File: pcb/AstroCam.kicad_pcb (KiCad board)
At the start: 2 copper layers, 40 x 40 mm, 93 parts, among them P1 CONN_01X02, P10 CONN_01X14, P2 CONN_01X18, P3 CONN_01X18, P4 CONN_01X04, P5 CONN_01X01, P8 CONN_01X06, P9 CONN_01X02, Q1 2SC5095, Q2 MT3S20TU, Q3 2SC5095, Q4 MT3S20TU, U1 TPS2420, U10 ICX825AQA, U11 ADDI7013, U2 LT3487, U3 TPS63002, U4 TXB0104, U7 TPS56x200, U8 LMZ10500, U9 CXD3400N

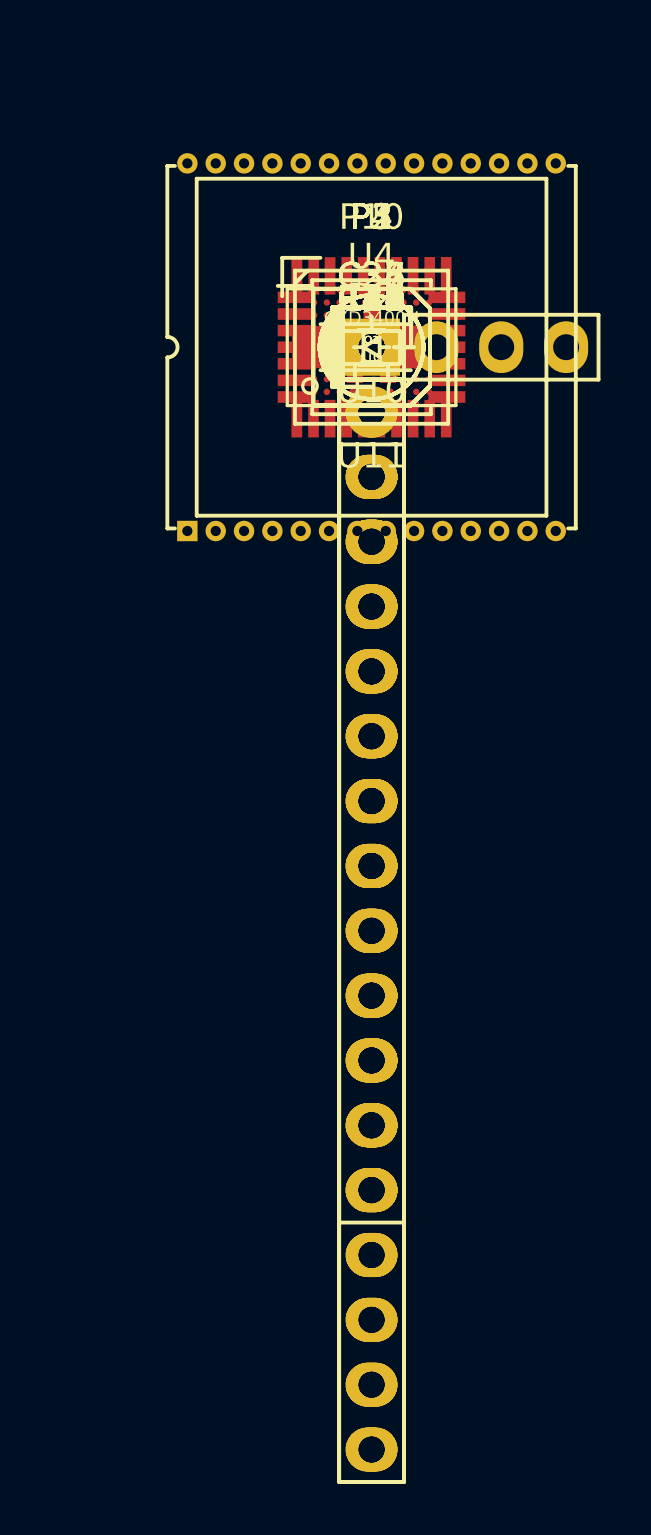
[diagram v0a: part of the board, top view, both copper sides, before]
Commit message: Cleanups
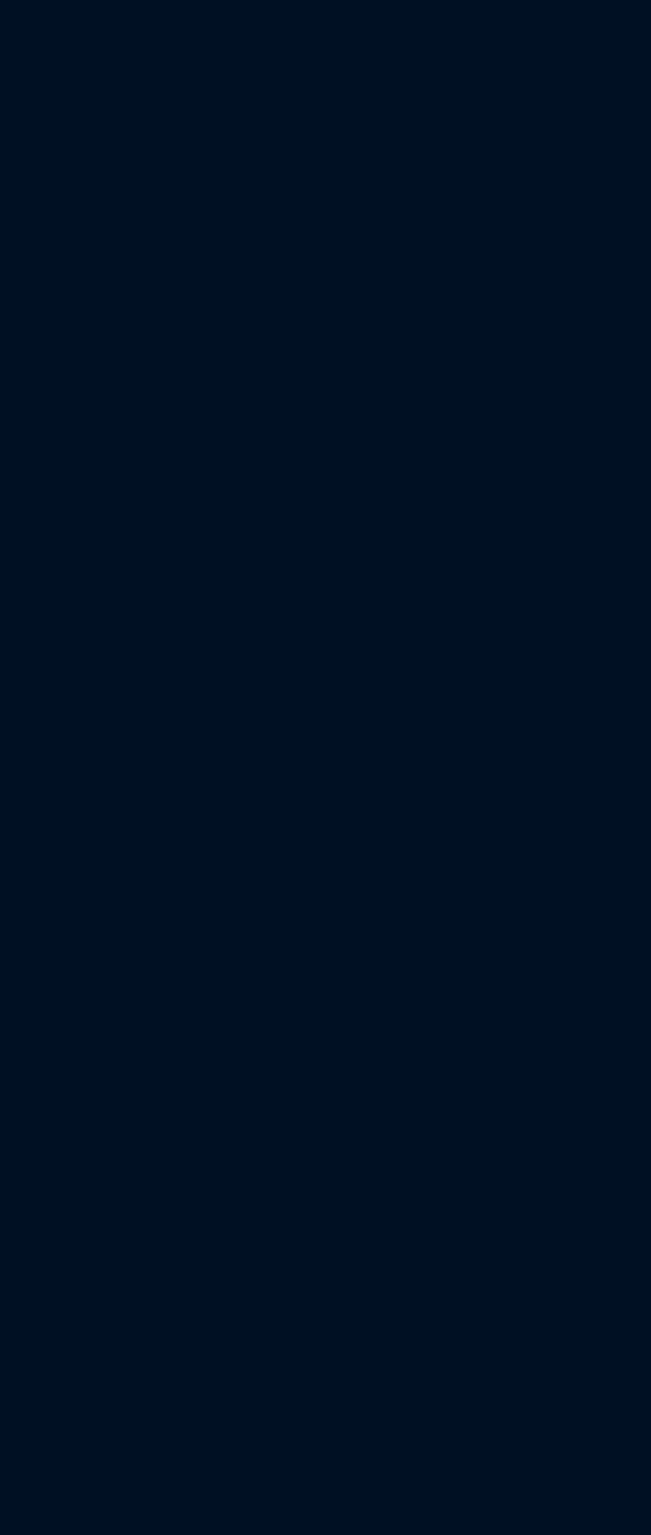
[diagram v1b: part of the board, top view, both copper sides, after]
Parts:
- removed C12, C13, C26, C27: 0.1u, Capacitors_SMD:C_0603
- removed C28: 1u/35V, Capacitors_SMD:c_elec_4x5.3
- removed C29: 0.1uF, Capacitors_SMD:C_0603
- removed C30: 2200pF, Capacitors_SMD:C_0603
- removed C31, C32: 0.1, Capacitors_SMD:C_0603
- removed C33, C35: 0.01, Capacitors_SMD:C_0603
- removed C34, C36, C37: 3.3/20V, Capacitors_SMD:c_elec_4x5.3
- removed C38, C39, C40, C41, C42, C43, C44, C45, C46: 0.1uF, Capacitors_SMD:C_0603_HandSoldering
- removed C47: 4.7uF, Capacitors_SMD:C_0603_HandSoldering
- removed C48, C49: 0.1u, Capacitors_SMD:C_0603_HandSoldering
- removed D2: D, Diodes_SMD:SOD-123
- removed P1: CONN_01X02, Pin_Headers:Pin_Header_Straight_1x02
- removed P10: CONN_01X14, Pin_Headers:Pin_Header_Straight_1x14
- removed P2, P3: CONN_01X18, Pin_Headers:Pin_Header_Straight_1x18
- removed P4: CONN_01X04, Socket_Strips:Socket_Strip_Straight_1x04
- removed P5: CONN_01X01, Socket_Strips:Socket_Strip_Straight_1x01
- removed Q1, Q3: 2SC5095, w_smd_trans:sot323
- removed Q2, Q4: MT3S20TU, w_smd_trans:sot323
- removed R10, R11, R14, R15: 10K, Resistors_SMD:R_0603_HandSoldering
- removed R12, R20: 1.17K, Resistors_SMD:R_0603_HandSoldering
- removed R13, R21: 1.74K, Resistors_SMD:R_0603_HandSoldering
- removed R18: 100k, Resistors_SMD:R_0603_HandSoldering
- removed R19: 1M0, Resistors_SMD:R_0603_HandSoldering
- removed R22: 10.0k, Resistors_SMD:R_0603_HandSoldering
- removed U10: ICX825AQA, camera:ICX825
- removed U11: ADDI7013, camera:csp-bga-bc-76-3
- removed U4: TXB0104, Housings_SSOP:TSSOP-14_4.4x5mm_Pitch0.65mm
- removed U9: CXD3400N, w_smd_dil:tssop-20

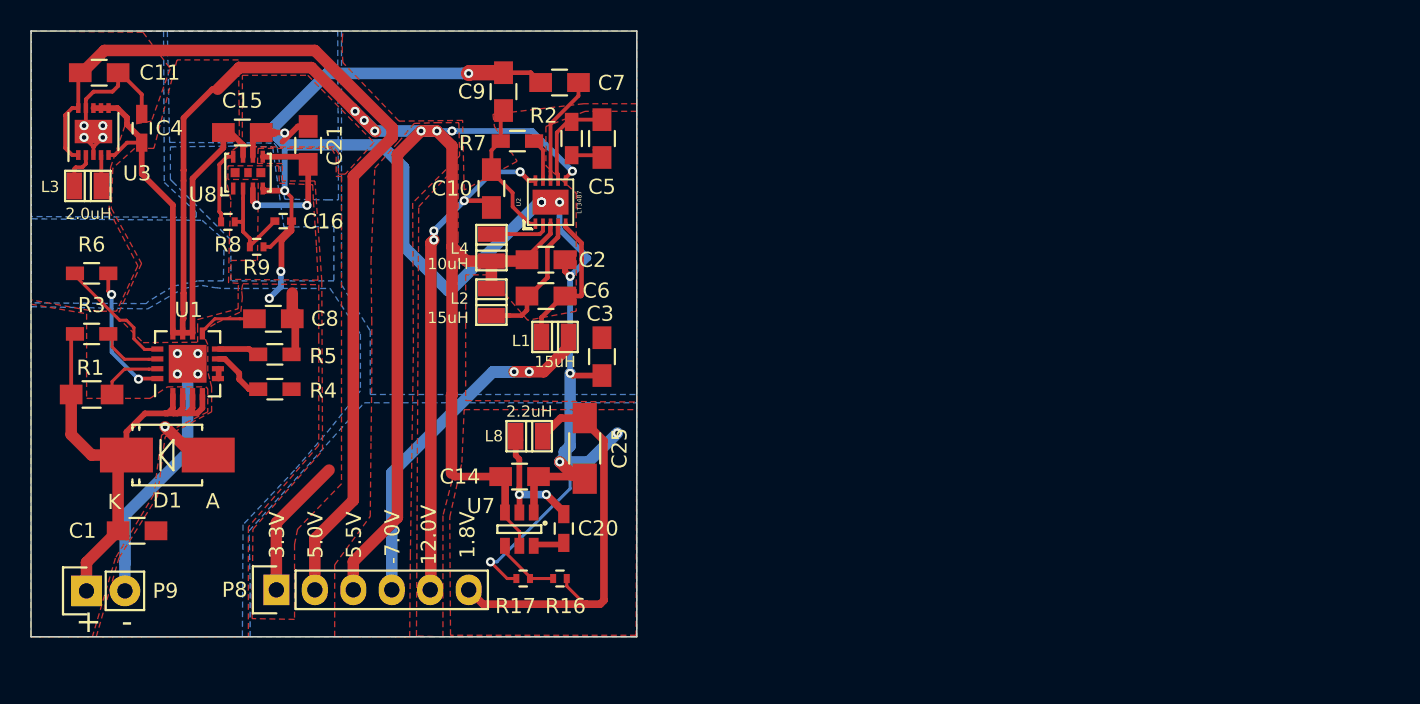
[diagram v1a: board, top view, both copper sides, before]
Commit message: Latest, greatest.
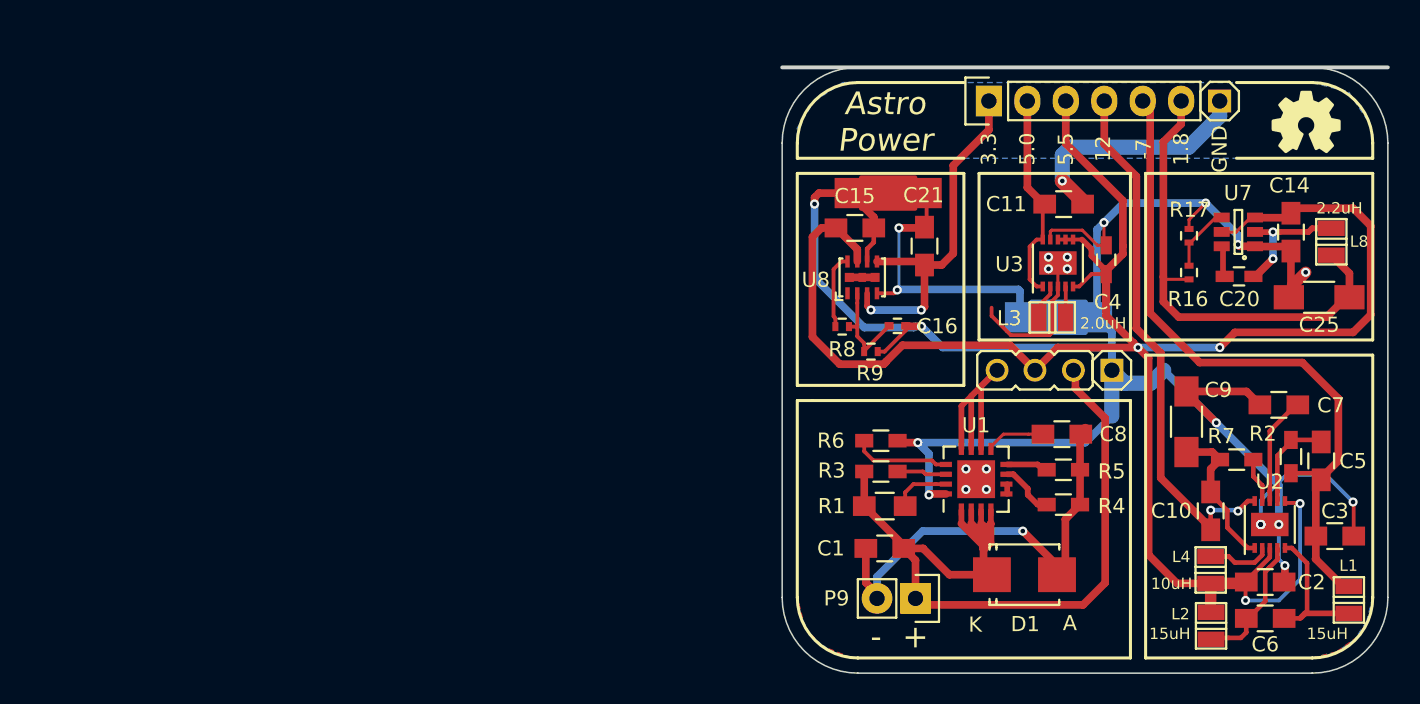
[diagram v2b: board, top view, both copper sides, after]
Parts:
- added ?: , xess:oshw-logo2, F.Cu at (179.6, 68.6)
- added JP5: JUMPER3, xess:xess-JP2, F.Cu at (161.7, 85.0)
- added P11: CONN_01X01, xess:HDR_1x1, F.Cu at (166.8, 85.0)
- added P12: CONN_01X01, xess:HDR_1x1, F.Cu at (173.9, 67.2)
- added T1: NET-TIE, Oddities:NetTie-I_Connected_SMD, B.Cu at (163.2, 81.5)
- added T2: NET-TIE, Oddities:NetTie-I_Connected_SMD, F.Cu at (152.0, 73.3)
- C9: footprint Capacitors_SMD:C_0805_HandSoldering -> Capacitors_SMD:C_1206_HandSoldering
- D1: footprint Diodes_SMD:Diode-SMB_Handsoldering -> Diodes_SMD:SMB_Standard
- U2: footprint w_smd_qfn:dfn10-3x3 -> Housings_DFN_QFN:DFN-10-1EP_3x3mm_Pitch0.5mm
- U8: footprint camera:llp-8 -> engstad:llp-8
- moved C4 64.3 mm to (166.4, 77.7)
- moved U3 64.3 mm to (163.2, 77.9)
- moved C11 64.3 mm to (163.6, 74.0)
- moved L3 64.3 mm to (162.8, 81.5)
- moved D1 57.1 mm to (161.0, 98.5)
- moved P8 57.1 mm to (158.7, 67.2)
- moved L1 55.2 mm to (182.4, 100.2), turned to 270 degrees
- moved P9 54.7 mm to (153.8, 100.1), turned to 270 degrees
- moved L8 54.5 mm to (181.3, 76.5), turned to 270 degrees
- moved C14 53.4 mm to (178.6, 75.9), turned to 270 degrees
- moved R6 53.3 mm to (151.5, 89.7)
- moved R3 52.9 mm to (151.5, 91.7)
- moved R1 52.9 mm to (151.8, 94.0)
- moved U1 52.6 mm to (157.8, 92.2)
- moved C8 52.6 mm to (163.5, 89.2)
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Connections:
- net /power-supply/V_BAT renamed VIN*
- C11 pad 2: GND -> /power-supply/PGND
- C21 pad 2: GND -> /power-supply/PGND
- P8 pad 4: /power-supply/-7V -> /power-supply/+12V
- P8 pad 5: /power-supply/+12V -> /power-supply/-7V
- U1 pad 10: /power-supply/5V5 -> /power-supply/OUT_5V5
- U1 pad 11: /power-supply/5V5 -> /power-supply/OUT_5V5
- U1 pad 12: /power-supply/5V5 -> /power-supply/OUT_5V5
- U3 pad 11: GND -> /power-supply/PGND
- U3 pad 3: GND -> /power-supply/PGND
- U8 pad 4: GND -> /power-supply/PGND
- U8 pad 9: GND -> Net-(U8-Pad9)
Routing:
- net /power-supply/PGND: track 0.00 -> 50.6 mm, vias 0 -> 7
- net /power-supply/5V0: track 63.0 -> 14.1 mm
- net (no net): track 0.00 -> 40.0 mm
- net VIN*: track 33.7 -> 57.4 mm
- net /power-supply/5V5: track 160.3 -> 137.3 mm, vias 7 -> 4
- net /power-supply/OUT_5V5: track 0.00 -> 17.7 mm
- net /power-supply/-7V: track 29.2 -> 46.2 mm, vias 2 -> 0
- net GND: track 164.6 -> 172.2 mm, vias 25 -> 20
- net /power-supply/1V8: track 27.5 -> 32.0 mm
- net /power-supply/3V3: track 19.8 -> 24.2 mm
- net Net-(R6-Pad1): track 8.25 -> 6.45 mm
- net Net-(U8-Pad9): track 0.00 -> 1.70 mm
- net /power-supply/+12V: track 34.3 -> 35.7 mm, vias 4 -> 2
- net Net-(R3-Pad2): track 4.23 -> 3.27 mm
- net /power-supply/CAP: track 9.31 -> 9.98 mm
- added copper zone on B.Cu, net /power-supply/PGND
- added copper zone on F.Cu, net /power-supply/PGND
- removed copper zone on F.Cu, net /power-supply/+12V
- removed copper zone on F.Cu, net /power-supply/-7V
- removed copper zone on F.Cu, net /power-supply/3V3
- removed copper zone on F.Cu, net /power-supply/5V5
- removed copper zone on F.Cu, net VIN*
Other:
- outline, holes or cut-outs redrawn
- net class Power added: clearance 0.1524, trace_width 0.508, via_dia 0.604774, via_drill 0.299974
- board text added: "-7"
- board text added: "1.8"
- board text added: "12"
- board text added: "3.3"
- board text added: "5.0"
- board text added: "5.5"
- board text added: "Astro Power"
- board text added: "GND"
- board text removed: "-7.0V"
- board text removed: "1.8V"
- board text removed: "12.0V"
- board text removed: "3.3V"
- board text removed: "5.0V"
- board text removed: "5.5V"
